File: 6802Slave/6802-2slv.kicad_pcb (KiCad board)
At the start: 2 copper layers, 68 parts, among them J1 DB15, J2 USB B conn., J3 USB A connector, J4 ICSP, P1 CONN_1, U1 LTC6802-2, U2 TCLT1009, U3 ACPL-W61L, U4 ACPL-K64L, U5 PIC16F1825, U6 MAX232

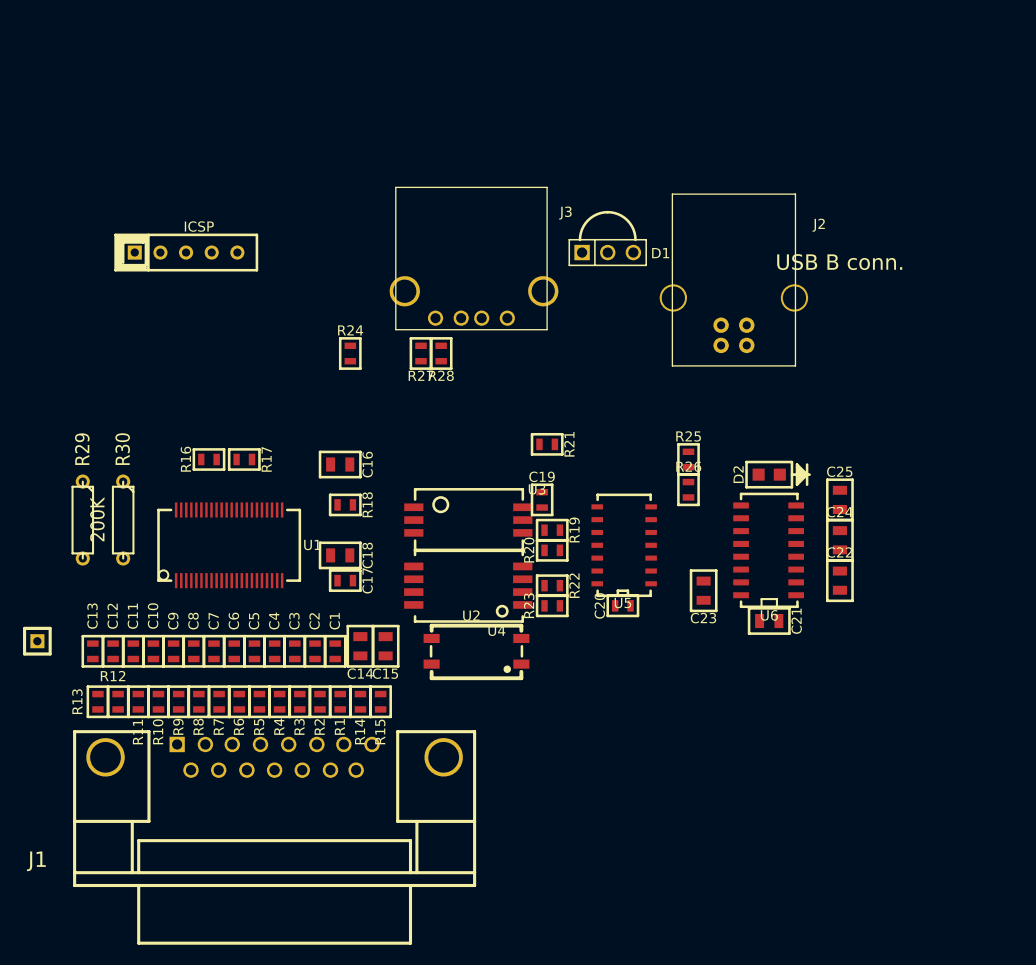
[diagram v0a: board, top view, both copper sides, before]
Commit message: layout work
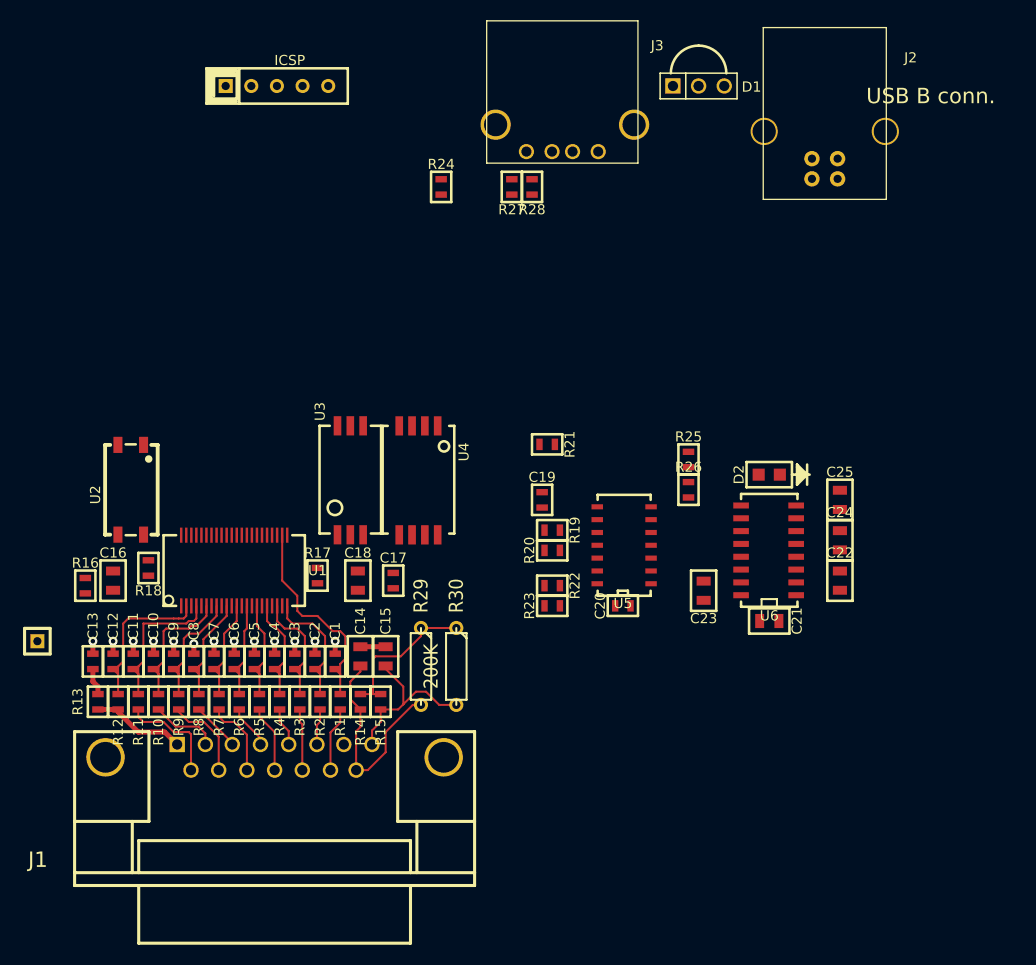
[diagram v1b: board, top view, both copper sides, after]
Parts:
- moved U2 37.8 mm to (208.2, 194.5), turned to 270 degrees
- moved R29 36.5 mm to (237.0, 212.0)
- moved R30 36.0 mm to (240.5, 212.0)
- moved C16 25.3 mm to (206.5, 203.5), turned to 270 degrees
- moved R18 20.5 mm to (210.0, 202.2), turned to 90 degrees
- moved D1 18.8 mm to (264.5, 154.5)
- moved J2 18.8 mm to (277.0, 159.0)
- moved J3 18.8 mm to (251.0, 161.0)
- moved J4 18.8 mm to (224.0, 154.5)
- moved R24 18.8 mm to (239.0, 164.5)
- moved R27 18.8 mm to (246.0, 164.5)
- moved R28 18.8 mm to (248.0, 164.5)
- moved R16 17.5 mm to (203.8, 204.0), turned to 270 degrees
- moved R17 13.6 mm to (226.8, 203.0), turned to 270 degrees
- moved U3 12.1 mm to (230.0, 193.8), turned to 0 degrees
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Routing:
- net N-0000065: track 0.00 -> 21.6 mm
- net N-0000014: track 0.00 -> 20.6 mm
- net GNDPWR: track 0.00 -> 18.3 mm, vias 0 -> 13
- net N-0000083: track 0.00 -> 17.1 mm
- net N-0000066: track 0.00 -> 15.5 mm
- net N-0000011: track 0.00 -> 15.5 mm
- net N-0000012: track 0.00 -> 14.6 mm
- net N-0000016: track 0.00 -> 13.0 mm
- net N-0000013: track 0.00 -> 12.4 mm
- net N-0000017: track 0.00 -> 11.6 mm
- net N-0000081: track 0.00 -> 11.5 mm
- net N-0000010: track 0.00 -> 10.6 mm
- net N-0000020: track 0.00 -> 10.5 mm
- net N-0000033: track 0.00 -> 10.2 mm
- net N-0000022: track 0.00 -> 10.2 mm
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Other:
- rule trace_min: 0.254 -> 0.2
